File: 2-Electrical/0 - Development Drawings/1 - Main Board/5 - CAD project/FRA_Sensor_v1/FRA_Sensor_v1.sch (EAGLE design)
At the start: 141 parts, among them IC1 CP2101, IC2 LMV611, IC3 TS520533, J2 ETH_CONN, J3 USB, Q1 Si2300DS, Q2 FDN306P, T1 BC847, T2 BC847, T3 BC847, U2 ESP-WROOM-32, X1 TB001-500-02BE, Y3 32.768kHz

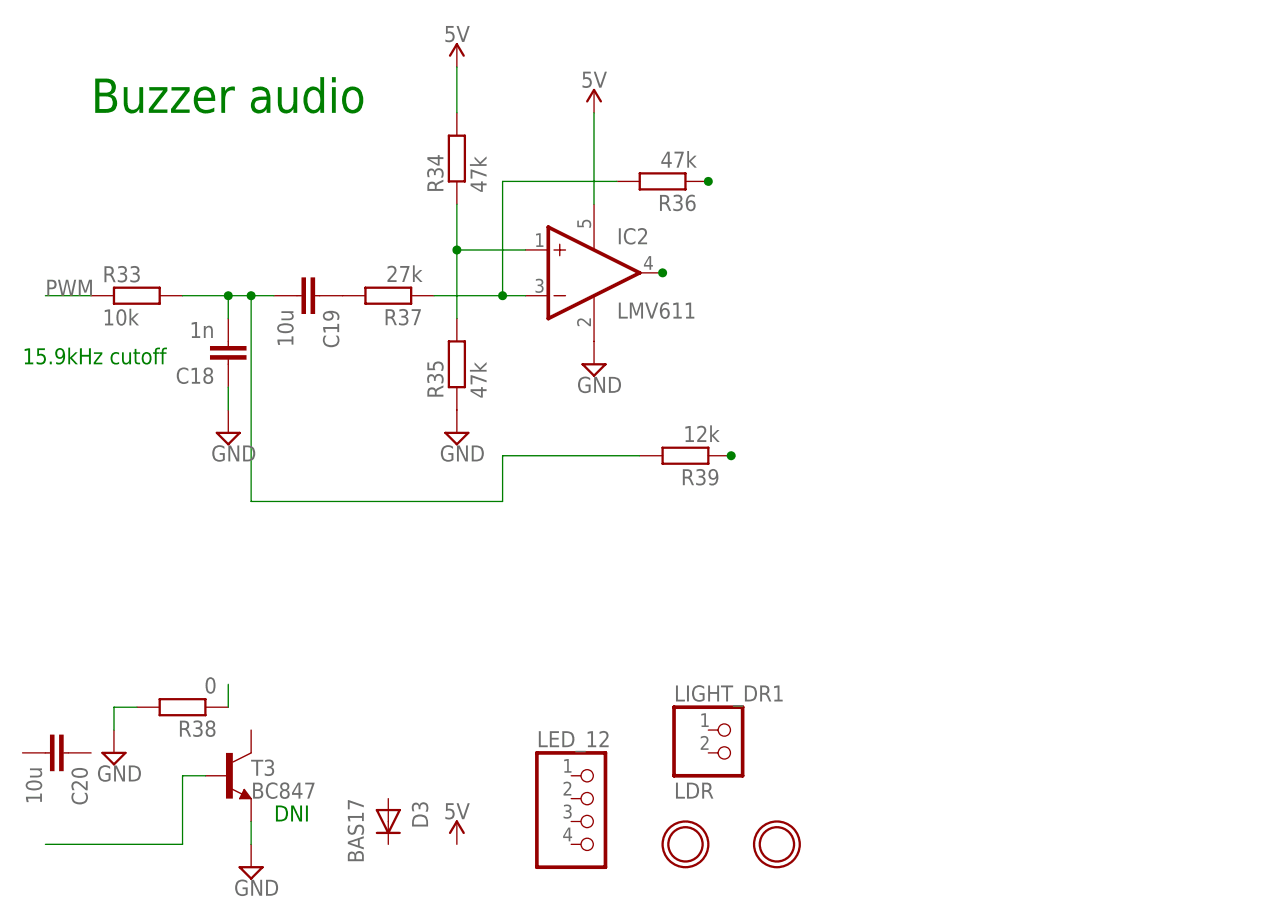
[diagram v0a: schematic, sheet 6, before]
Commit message: placment drafts
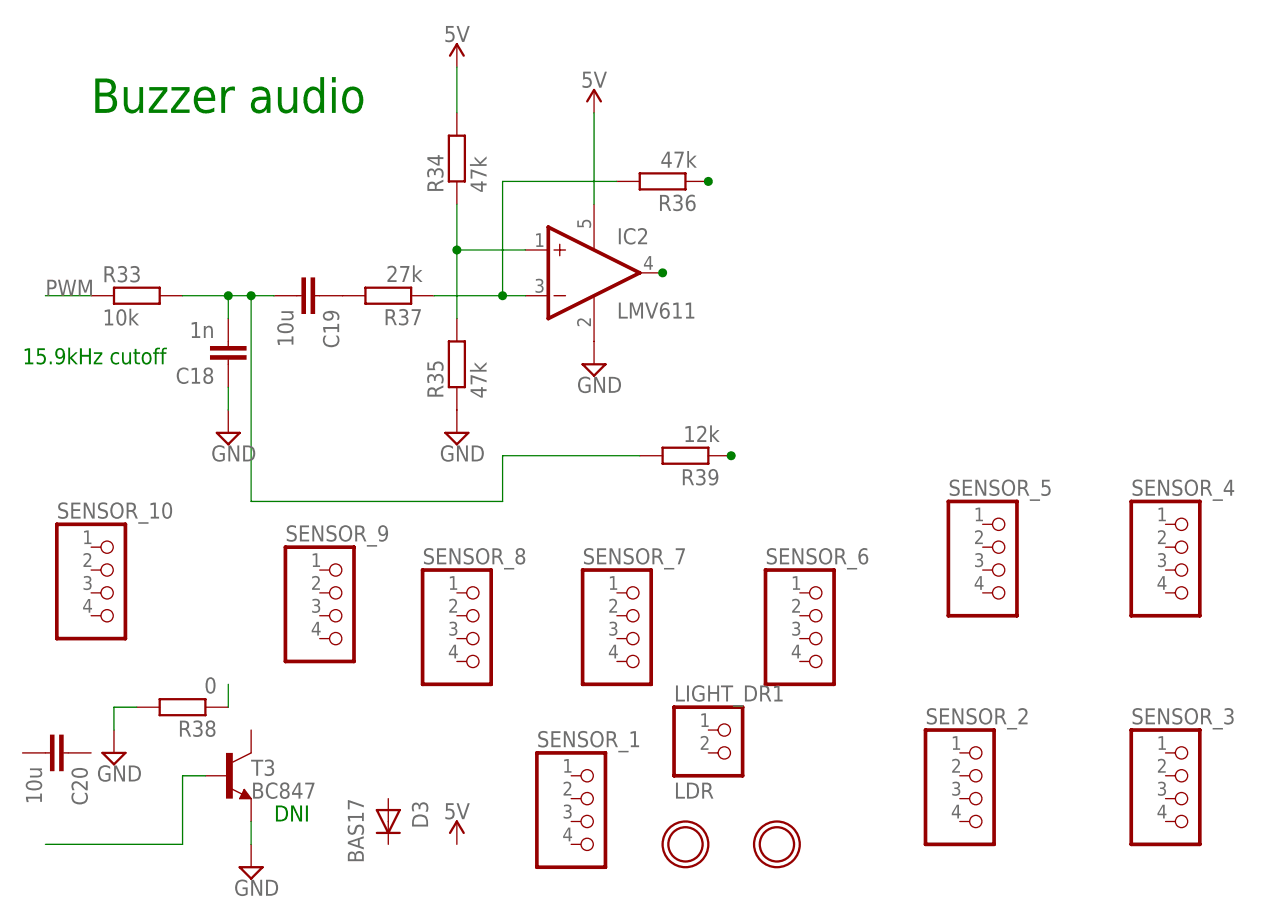
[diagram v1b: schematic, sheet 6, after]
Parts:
- added SENSOR_10, SENSOR_2, SENSOR_3, SENSOR_4, SENSOR_5, SENSOR_6, SENSOR_7, SENSOR_8, SENSOR_9: SENS1, pinhead:PINHD-1X4
- SENSOR_1: value LED_ring_12 -> SENS1
- renumbered LED_12 to SENSOR_1
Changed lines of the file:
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@@
 <part name="R21" library="resistor" deviceset="R-EU_" device="R0603" value="0"/>
 <part name="D3" library="nxp_60" deviceset="BAS17" device=""/>
-<part name="LED_12" library="pinhead" deviceset="PINHD-1X4" device="" value="LED_ring_12"/>
+<part name="SENSOR_1" library="pinhead" deviceset="PINHD-1X4" device="" value="SENS1"/>
 <part name="R25" library="resistor" deviceset="R-EU_" device="R0603" value="10K"/>
 <part name="C16" library="resistor" deviceset="C-EU" device="C0603K" value="1n"/>
@@
 <part name="SUPPLY54" library="supply2" deviceset="GND" device=""/>
 <part name="U$7" library="FRA_eagle_lib" deviceset="ETH_MODULE_OUTLINE" device=""/>
+<part name="SENSOR_2" library="pinhead" deviceset="PINHD-1X4" device="" value="SENS1"/>
+<part name="SENSOR_3" library="pinhead" deviceset="PINHD-1X4" device="" value="SENS1"/>
+<part name="SENSOR_4" library="pinhead" deviceset="PINHD-1X4" device="" value="SENS1"/>
+<part name="SENSOR_5" library="pinhead" deviceset="PINHD-1X4" device="" value="SENS1"/>
+<part name="SENSOR_6" library="pinhead" deviceset="PINHD-1X4" device="" value="SENS1"/>
+<part name="SENSOR_7" library="pinhead" deviceset="PINHD-1X4" device="" value="SENS1"/>
+<part name="SENSOR_8" library="pinhead" deviceset="PINHD-1X4" device="" value="SENS1"/>
+<part name="SENSOR_9" library="pinhead" deviceset="PINHD-1X4" device="" value="SENS1"/>
+<part name="SENSOR_10" library="pinhead" deviceset="PINHD-1X4" device="" value="SENS1"/>
 </parts>
 <sheets>
@@
 <instance part="SUPPLY85" gate="G$1" x="53.34" y="86.36"/>
 <instance part="D3" gate="G$1" x="30.48" y="7.62" rot="R270"/>
-<instance part="LED_12" gate="A" x="53.34" y="7.62" smashed="yes">
+<instance part="SENSOR_1" gate="A" x="53.34" y="7.62" smashed="yes">
 <attribute name="NAME" x="46.99" y="15.875" size="1.778" layer="95"/>
 </instance>
@@
 <instance part="U$6" gate="G$1" x="63.5" y="5.08"/>
 <instance part="LIGHT_DR1" gate="G$1" x="68.58" y="15.24"/>
+<instance part="SENSOR_2" gate="A" x="96.52" y="10.16" smashed="yes">
+<attribute name="NAME" x="90.17" y="18.415" size="1.778" layer="95"/>
+</instance>
+<instance part="SENSOR_3" gate="A" x="119.38" y="10.16" smashed="yes">
+<attribute name="NAME" x="113.03" y="18.415" size="1.778" layer="95"/>
+</instance>
+<instance part="SENSOR_4" gate="A" x="119.38" y="35.56" smashed="yes">
+<attribute name="NAME" x="113.03" y="43.815" size="1.778" layer="95"/>
+</instance>
+<instance part="SENSOR_5" gate="A" x="99.06" y="35.56" smashed="yes">
+<attribute name="NAME" x="92.71" y="43.815" size="1.778" layer="95"/>
+</instance>
+<instance part="SENSOR_6" gate="A" x="78.74" y="27.94" smashed="yes">
+<attribute name="NAME" x="72.39" y="36.195" size="1.778" layer="95"/>
+</instance>
+<instance part="SENSOR_7" gate="A" x="58.42" y="27.94" smashed="yes">
+<attribute name="NAME" x="52.07" y="36.195" size="1.778" layer="95"/>
+</instance>
+<instance part="SENSOR_8" gate="A" x="40.64" y="27.94" smashed="yes">
+<attribute name="NAME" x="34.29" y="36.195" size="1.778" layer="95"/>
+</instance>
+<instance part="SENSOR_9" gate="A" x="25.4" y="30.48" smashed="yes">
+<attribute name="NAME" x="19.05" y="38.735" size="1.778" layer="95"/>
+</instance>
+<instance part="SENSOR_10" gate="A" x="0" y="33.02" smashed="yes">
+<attribute name="NAME" x="-6.35" y="41.275" size="1.778" layer="95"/>
+</instance>
 </instances>
 <busses>
